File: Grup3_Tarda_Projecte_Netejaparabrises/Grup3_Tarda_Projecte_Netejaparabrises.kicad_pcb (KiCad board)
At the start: 4 copper layers, 162.4 x 126.5 mm, 89 parts, among them IC1 L78S05CV, IC2 PIC18F258-I_SO, J1 Screw_Terminal_01x02, J10 Screw_Terminal_01x02, J11 Screw_Terminal_01x02, J12 Screw_Terminal_01x02, J2 BOTONERA, J3 PROGRAMMING CON, J4 JP1, J5 DE9_Plug_MountingHoles, J6 DE9_Plug_MountingHoles, J7 CONEXIOSENSOR, J8 Screw_Terminal_01x02, J9 Screw_Terminal_01x02, K1 1393280-6, K2 1393280-6, K3 1393280-6, K4 1393280-6, K5 1393280-6, K6 1393280-6, K7 1393280-6, K8 1393280-6, K9 1393280-6, Q1 BC817-25_RF, Q2 BC817-25_RF, Q3 BC817-25_RF, Q4 BC817-25_RF, Q5 BC817-25_RF, Q6 BC817-25_RF, Q7 BC817-25_RF, U1 Value, U2 LM393, Y1 ABLS2-8.000MHZ-D4Y-T

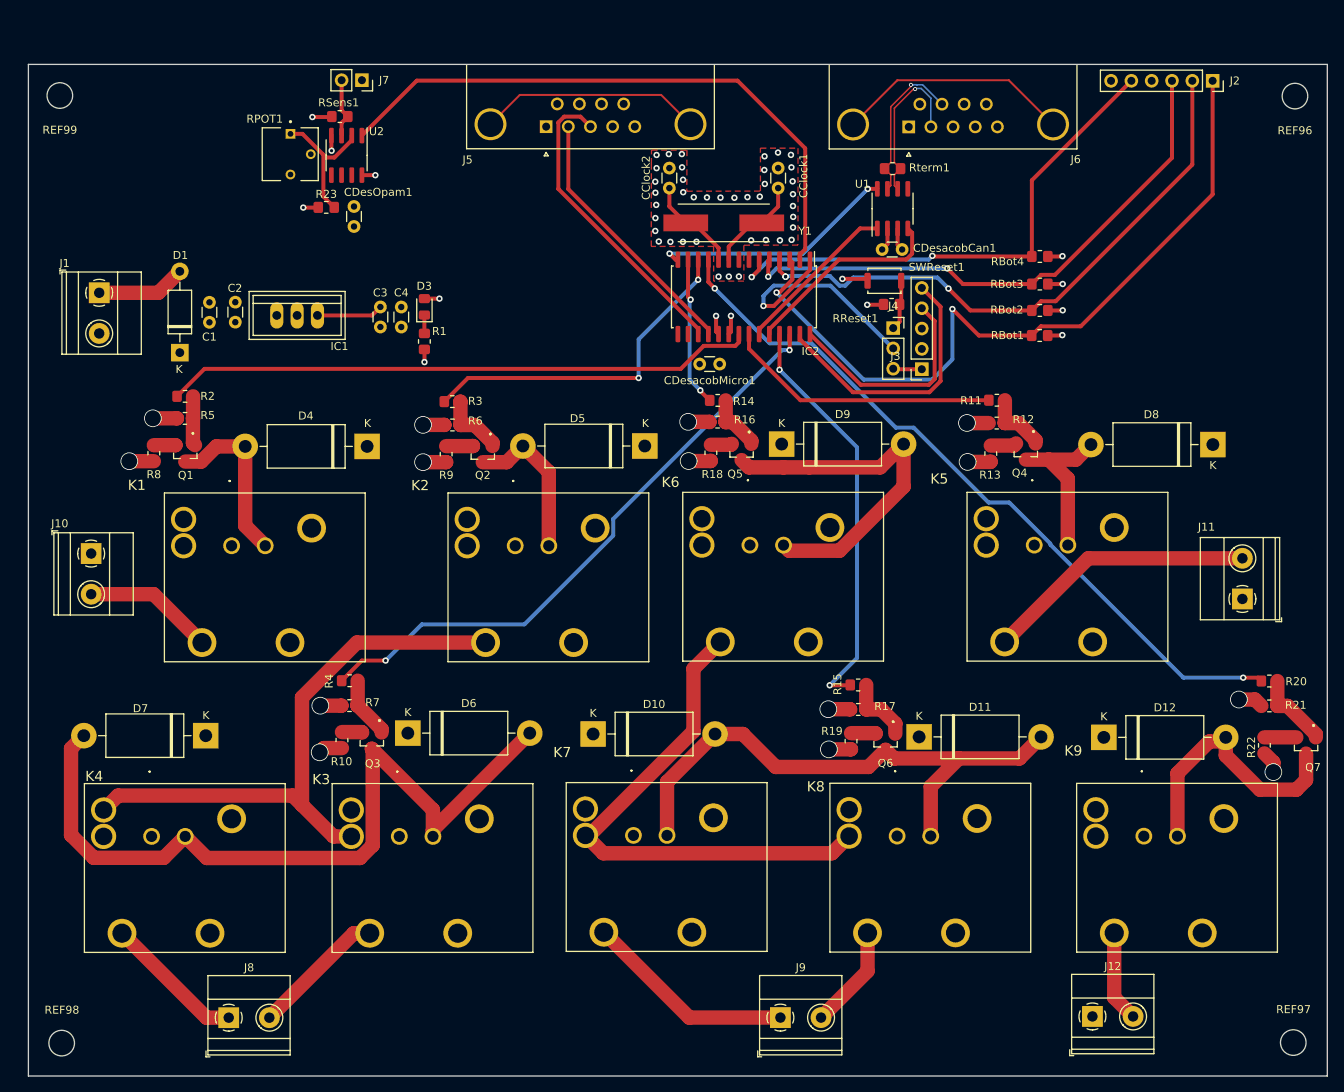
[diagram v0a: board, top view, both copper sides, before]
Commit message: canvis menors layout
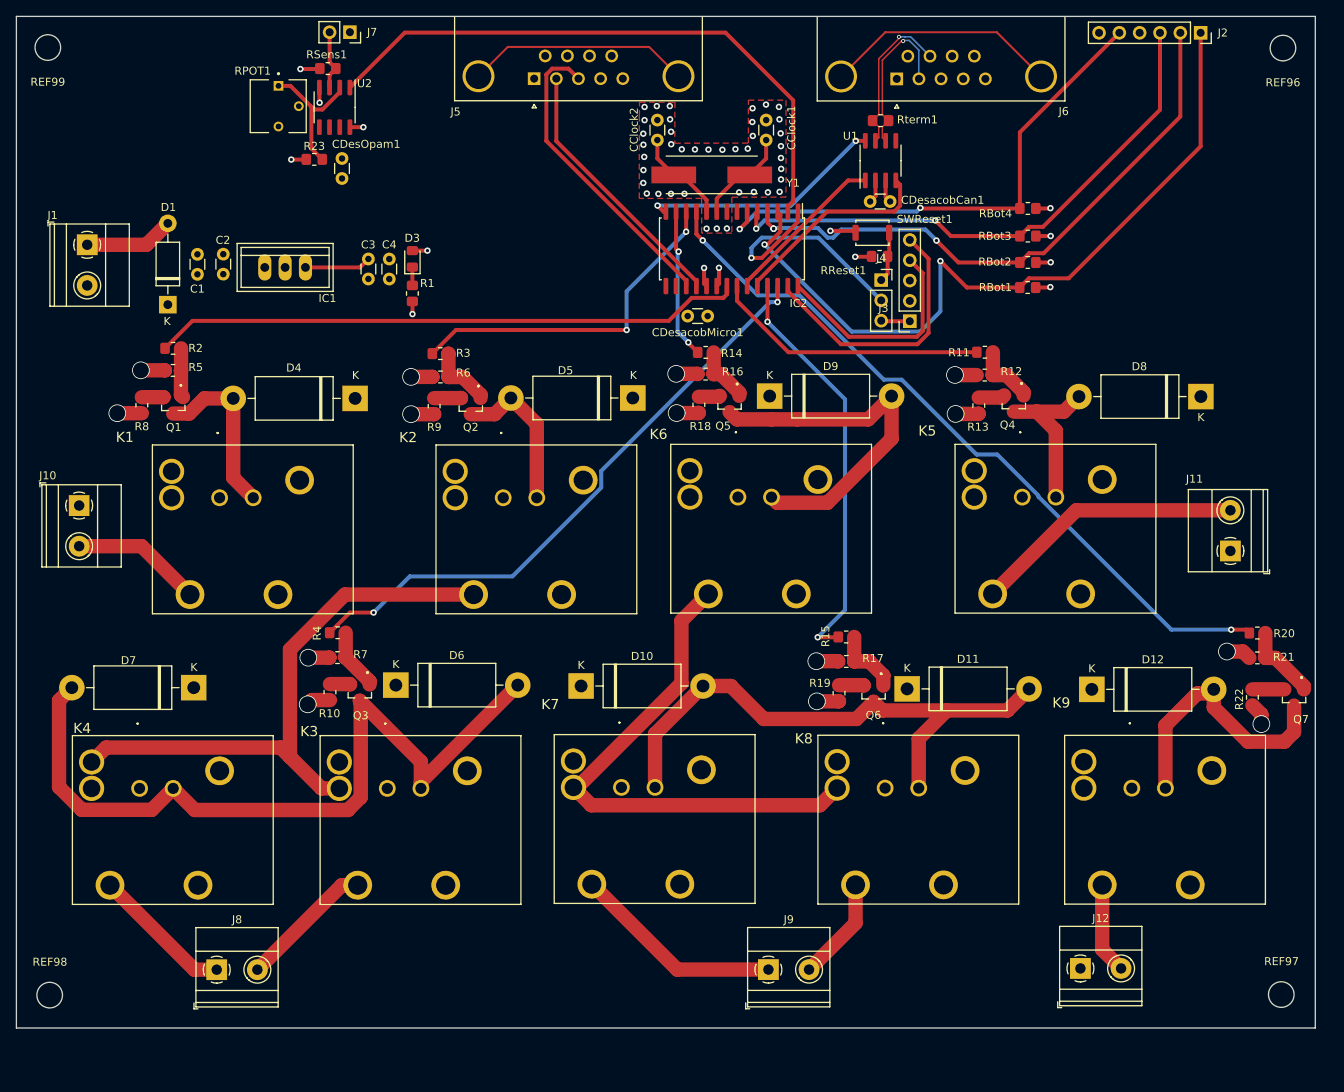
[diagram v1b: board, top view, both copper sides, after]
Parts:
- moved RBot1 6.18 mm to (186.6, 60.7)
- moved J2 6.18 mm to (208.2, 28.8)
- moved C1 6.18 mm to (82.8, 56.5)
- moved C2 6.18 mm to (86.0, 56.5)
- moved C3 6.18 mm to (104.2, 57.1)
- moved C4 6.18 mm to (106.8, 57.1)
- moved CClock1 6.18 mm to (153.9, 42.2)
- moved CClock2 6.18 mm to (140.3, 42.2)
- moved CDesOpam1 6.18 mm to (100.9, 44.5)
- moved CDesacobCan1 6.18 mm to (169.4, 49.9)
- moved CDesacobMicro1 6.18 mm to (146.6, 64.2)
- moved D10 6.18 mm to (130.8, 110.5)
- moved D11 6.18 mm to (171.5, 110.8)
- moved D12 6.18 mm to (194.6, 110.9)
- moved D3 6.18 mm to (109.7, 57.1)
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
